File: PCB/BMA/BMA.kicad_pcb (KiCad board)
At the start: 2 copper layers, 91.4 x 134.6 mm, 26 parts, among them J1 Conn_01x15, J10 Conn_01x10, J11 Conn_01x05, J12 Conn_01x04, J13 Conn_01x05, J14 Conn_01x05, J2 Conn_01x02, J3 Conn_01x02, J4 Conn_01x05, J5 Conn_01x05, J6 Conn_01x12, J7 Conn_01x12, J8 Conn_01x05, J9 Conn_01x10, K1 G5LE-1, K10 G5LE-1, K11 G5LE-1, K12 G5LE-1, K2 G5LE-1, K3 G5LE-1, K4 G5LE-1, K5 G5LE-1, K6 G5LE-1, K7 G5LE-1, K8 G5LE-1, K9 G5LE-1

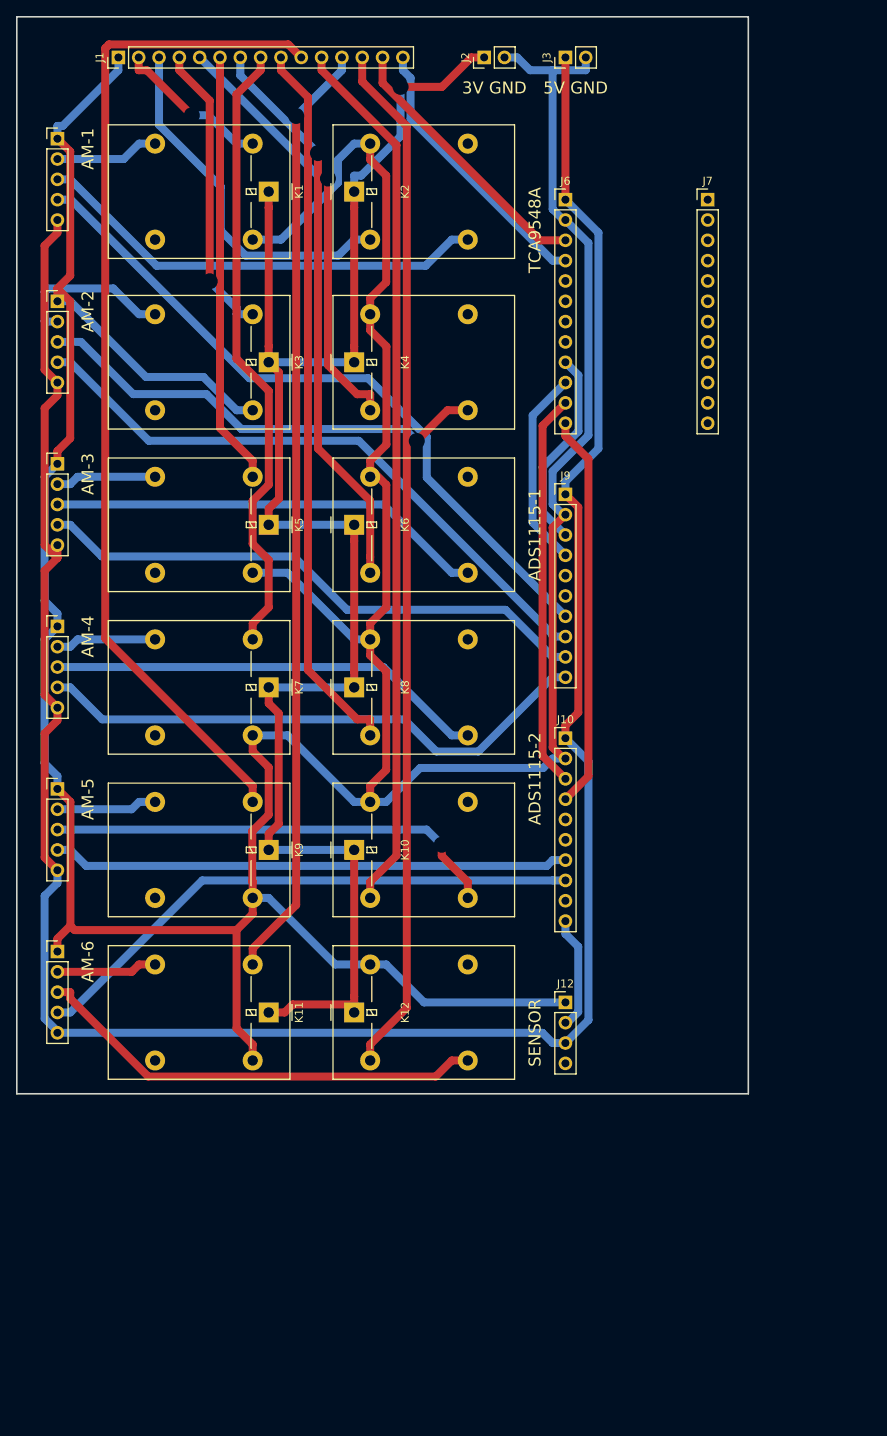
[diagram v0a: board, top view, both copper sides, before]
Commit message: POC 4
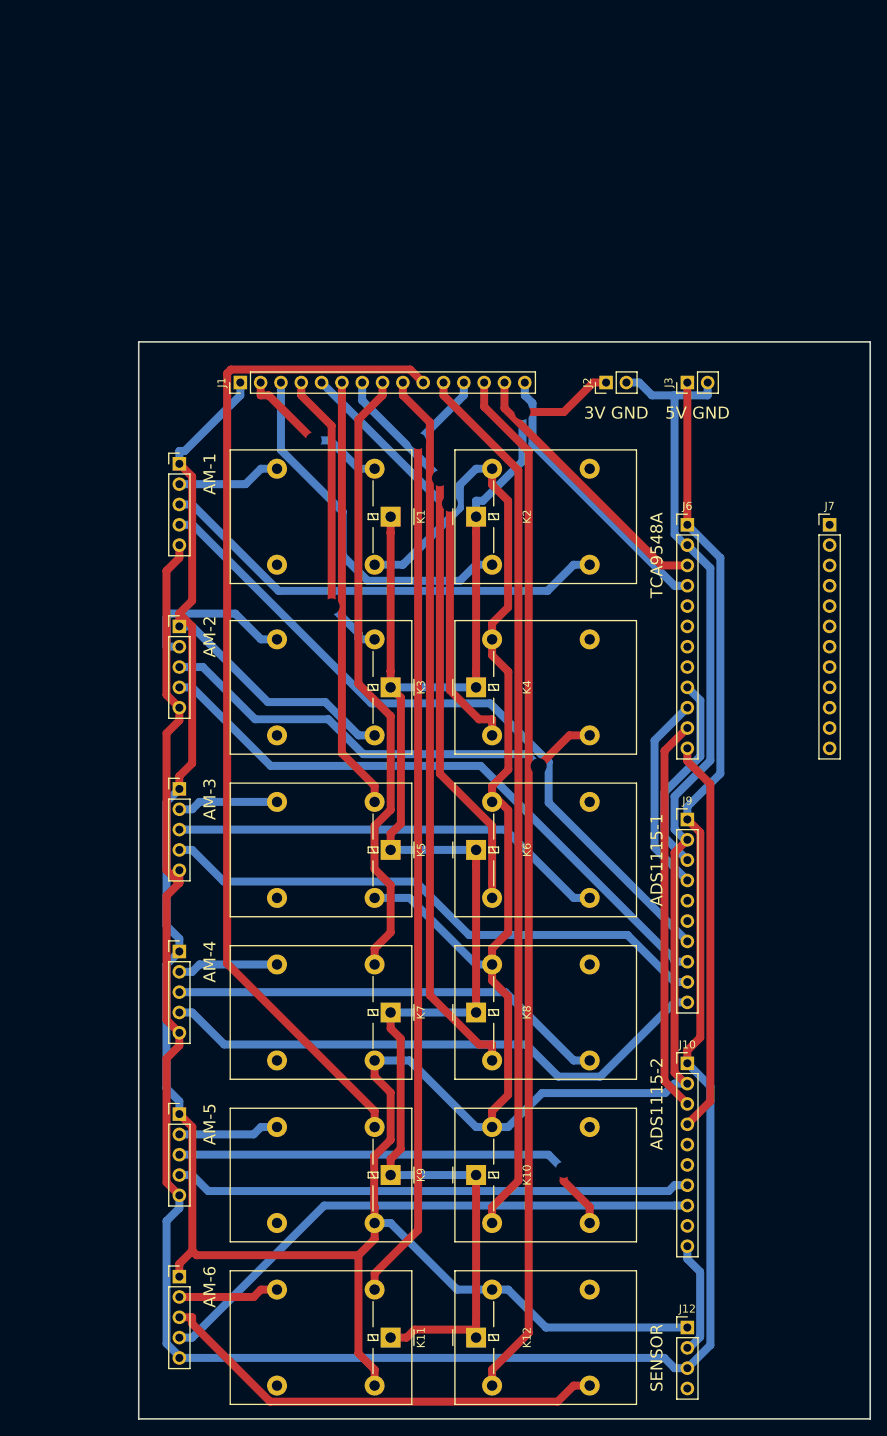
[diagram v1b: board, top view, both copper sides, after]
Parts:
- moved K1 43.4 mm to (92.4, 85.4)
- moved J10 43.4 mm to (129.5, 153.7)
- moved J13 43.4 mm to (66.0, 160.0)
- moved J14 43.4 mm to (66.0, 180.3)
- moved K11 43.4 mm to (92.4, 188.0)
- moved K12 43.4 mm to (103.1, 188.0)
- moved J5 43.4 mm to (66.0, 99.1)
- moved J8 43.4 mm to (66.0, 119.4)
- moved K2 43.4 mm to (103.1, 85.4)
- moved K3 43.4 mm to (92.4, 106.7)
- moved K5 43.4 mm to (92.4, 127.0)
- moved J1 43.4 mm to (73.7, 68.6)
- moved J2 43.4 mm to (119.4, 68.6)
- moved J3 43.4 mm to (129.5, 68.6)
- moved J4 43.4 mm to (66.0, 78.7)
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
